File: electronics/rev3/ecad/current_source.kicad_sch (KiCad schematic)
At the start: 27 parts, among them Q14 BSS84, U2 LM4030-2.5, U3 OPA4388IDR, U6 CD4066BM

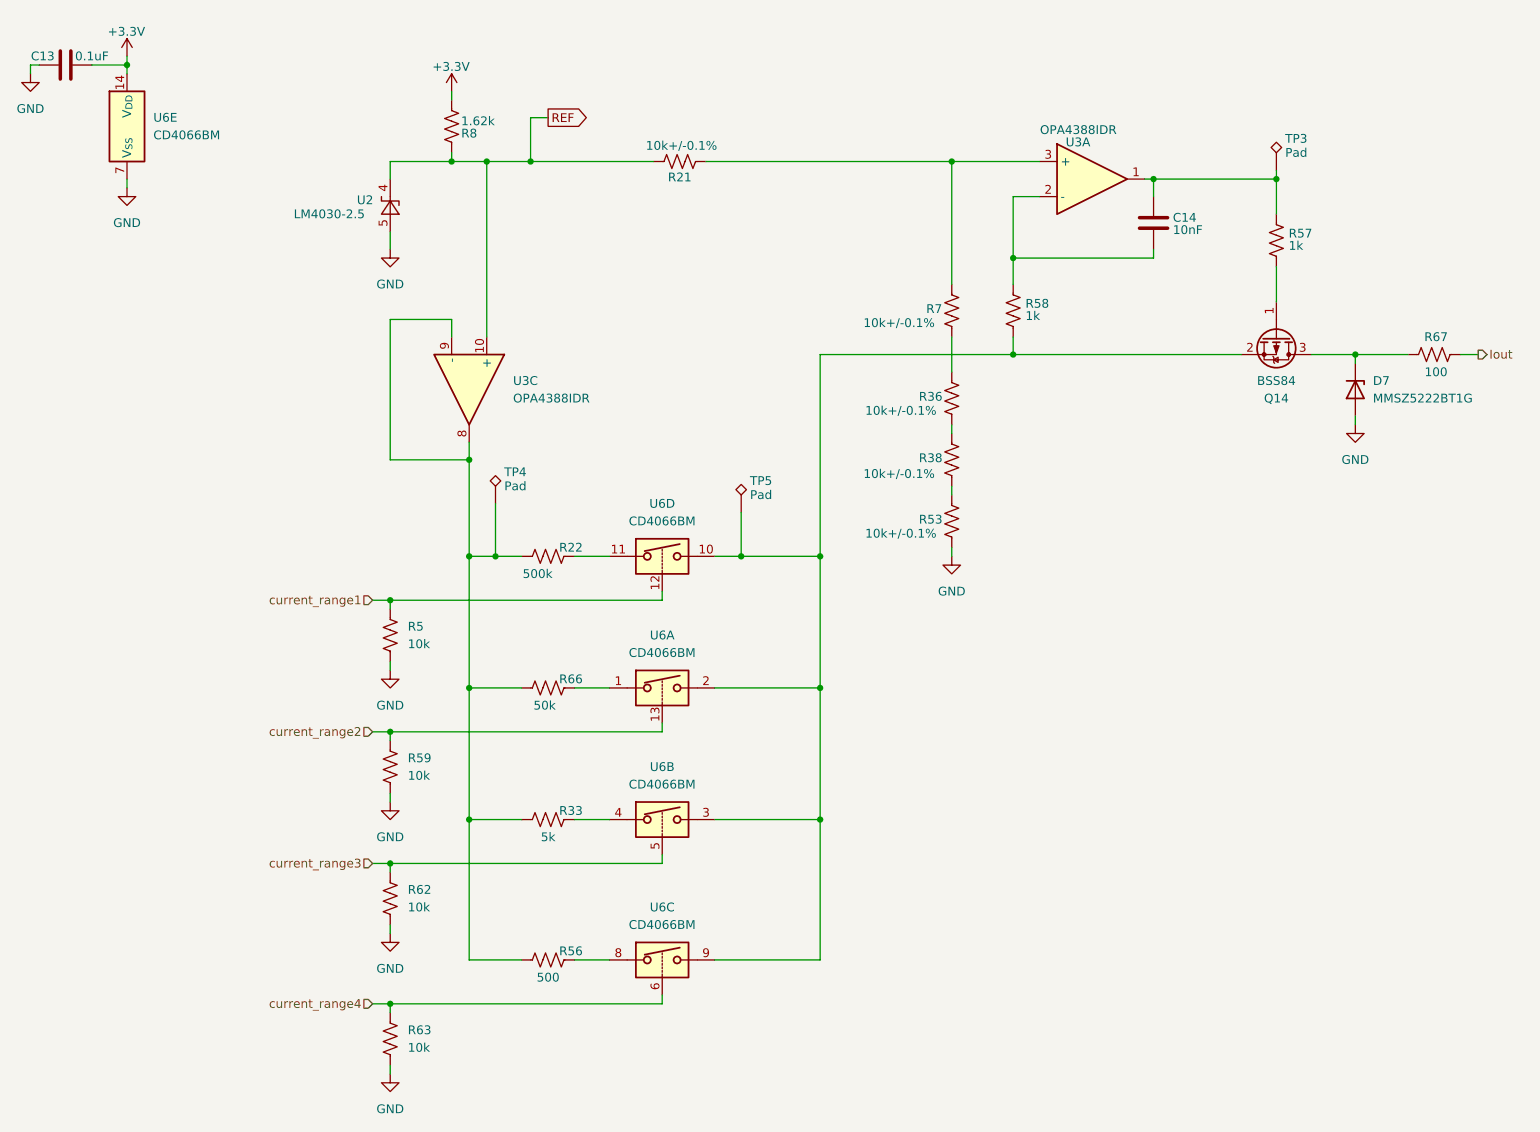
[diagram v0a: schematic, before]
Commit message: layout work rev3
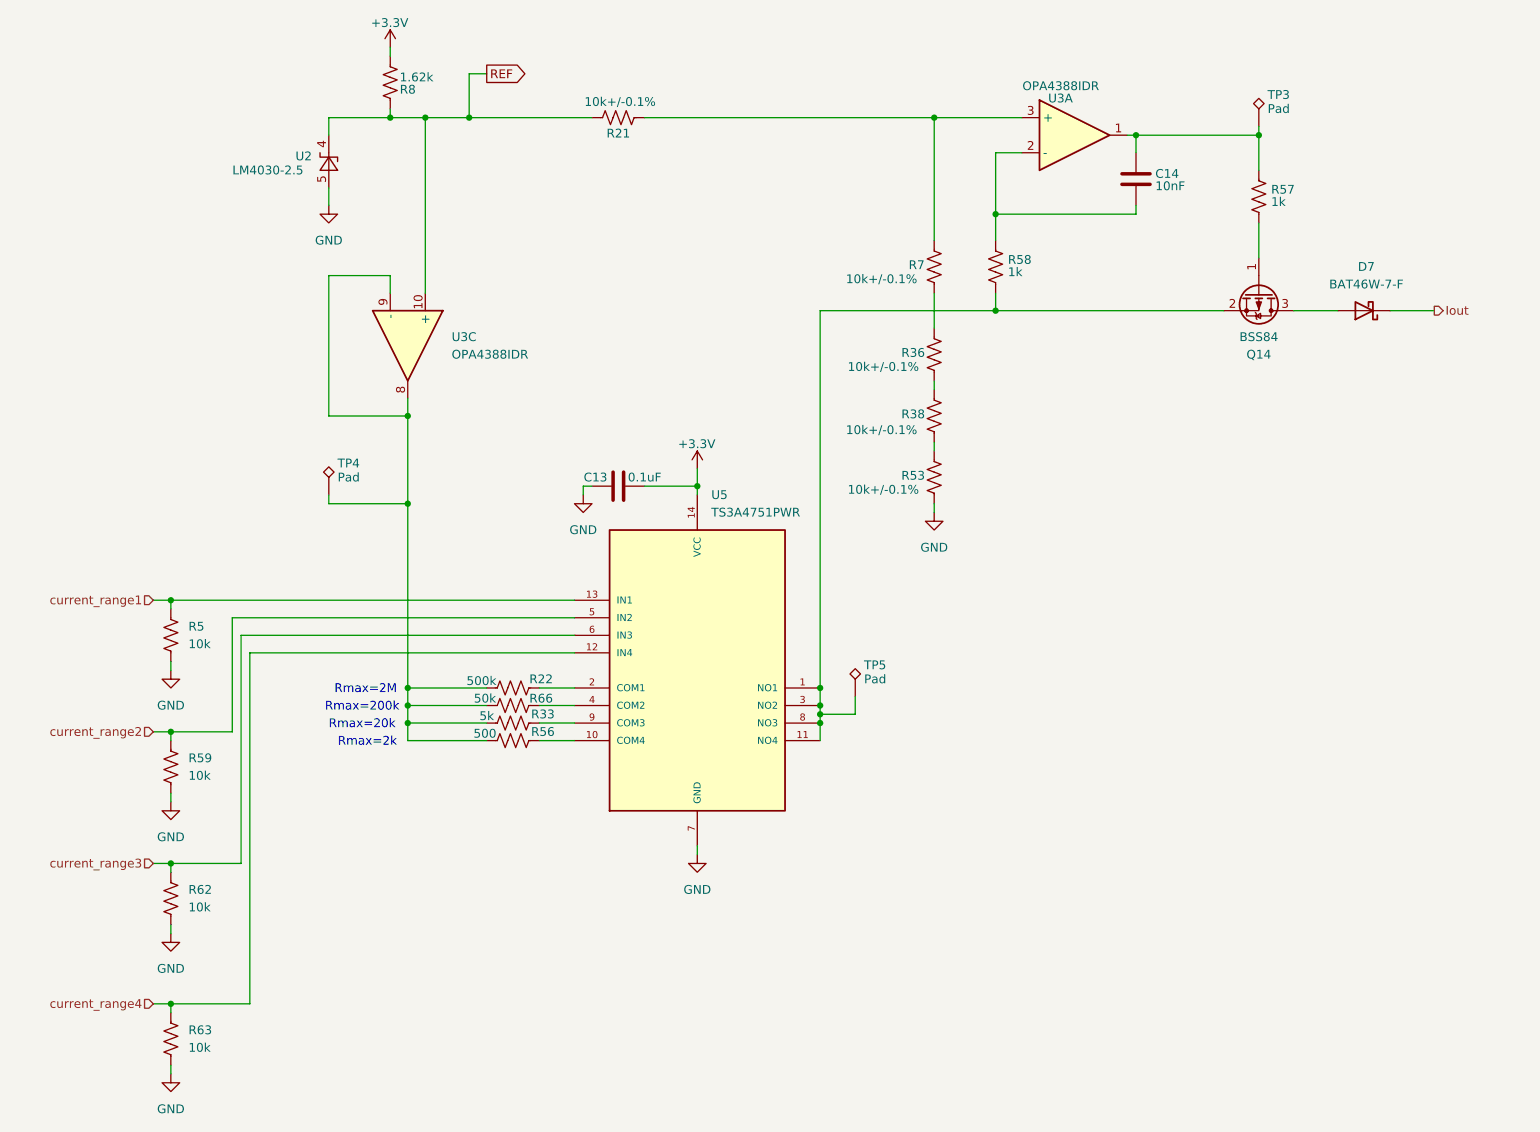
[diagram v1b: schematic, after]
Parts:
- removed D7: MMSZ5222BT1G, symbol Device:D_Zener
- removed R67: 100, Resistor_SMD:R_0805_2012Metric, symbol Device:R_US
- removed U6: CD4066BM, Package_SO:SO-14_3.9x8.65mm_P1.27mm, symbol Analog_Switch:CD4066BM
- added D7: BAT46W-7-F, Diode_SMD:D_SOD-123, symbol Device:D_Schottky
- added U5: TS3A4751PWR, Package_SO:TSSOP-14_4.4x5mm_P0.65mm, symbol multimeter_parts:TS3A4751PWR
- R21, R22, R33, R36, R38, R5, R7: footprint (none) -> Resistor_SMD:R_0805_2012Metric
- R8: footprint Resistor_SMD:R_0805_2012Metric_Pad1.20x1.40mm_HandSolder -> Resistor_SMD:R_0805_2012Metric
- U3: footprint (none) -> Package_SO:SOIC-14_3.9x8.7mm_P1.27mm
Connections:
- net +3.3V: now also U5.14 (VCC)
- net GND: now also U5.7 (GND)
- net Iout: now also D7.1 (K)
- net current_range1: now also U5.13 (IN1)
- net current_range2: now also U5.5 (IN2)
- net current_range3: now also U5.6 (IN3)
- net current_range4: now also U5.12 (IN4)
- net at R56.2: now also U5.10 (COM4)
- net at Q14.2 (S), R58.2, TP5.1: now also U5.1 (NO1), U5.11 (NO4), U5.3 (NO2), U5.8 (NO3)
- net at Q14.3 (D): now also D7.2 (A)
- net at R22.2: now also U5.2 (COM1)
- net at R66.2: now also U5.4 (COM2)
- net at R33.2: now also U5.9 (COM3)
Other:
- note added: "Rmax=200k"
- note added: "Rmax=20k"
- note added: "Rmax=2M"
- note added: "Rmax=2k"
- moved on the sheet: C13, C14, Q14, R21, R22, R33, R36, R38, R5, R53, R56, R57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

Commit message: layout complete
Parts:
- C13: Digikey Part # (none) -> 1276-1003-1-ND; Part # (none) -> CL21B104KBCNNNC; Unit Price (none) -> 0.1
- Q14: Digikey Part # (none) -> BSS84CT-ND; Part # (none) -> BSS84; Unit Price (none) -> 0.48
- R21, R36, R38, R53, R7: Digikey Part # (none) -> P10KDACT-ND; Part # (none) -> ERA-6AEB103V; Unit Price (none) -> 0.13
- R5, R59, R62, R63: Digikey Part # (none) -> RMCF0805FT10K0CT-ND; Part # (none) -> RMCF0805FT10K0; Unit Price (none) -> 0.1

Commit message: rev3 work
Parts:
- R57, R58: Digikey Part # (none) -> RMCF0805FT1K00CT-ND; Part # (none) -> RMCF0805FT1K00; Unit Price (none) -> 0.1
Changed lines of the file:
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@@
+			)
+		)
+		(property "Digikey Part #" "RMCF0805FT1K00CT-ND"
+			(at 163.83 54.61 0)
+			(effects
+				(font
+					(size 1.27 1.27)
+				)
+				(hide yes)
+			)
+		)
+		(property "Part #" "RMCF0805FT1K00"
+			(at 163.83 54.61 0)
+			(effects
+				(font
+					(size 1.27 1.27)
+				)
+				(hide yes)
+			)
+		)
+		(property "Unit Price" "0.1"
+			(at 163.83 54.61 0)
+			(effects
+				(font
+					(size 1.27 1.27)
+				)
+				(hide yes)
 			)
 		)
@@
 			(at 201.93 44.45 0)
 			(effects
+				(font
+					(size 1.27 1.27)
+				)
+				(hide yes)
+			)
+		)
+		(property "Digikey Part #" "RMCF0805FT1K00CT-ND"
+			(at 201.93 44.45 0)
+			(effects
+				(font
+					(size 1.27 1.27)
+				)
+				(hide yes)
+			)
+		)
+		(property "Part #" "RMCF0805FT1K00"
+			(at 201.93 44.45 0)
+			(effects
+				(font
+					(size 1.27 1.27)
+				)
+				(hide yes)
+			)
+		)
+		(property "Unit Price" "0.1"
+			(at 201.93 44.45 0)
+			(effects
